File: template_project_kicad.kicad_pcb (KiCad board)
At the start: 2 copper layers, 53.3 x 50.8 mm, 5 parts

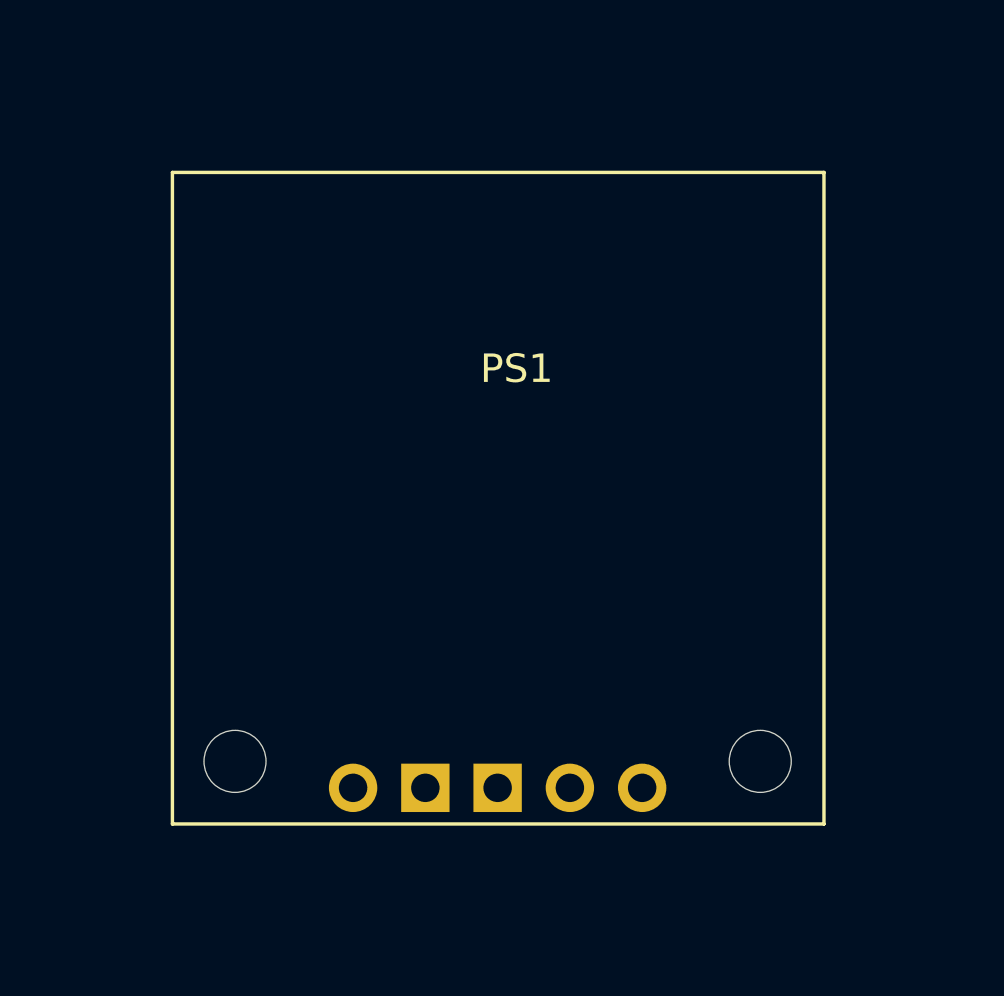
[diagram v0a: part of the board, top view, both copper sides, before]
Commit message: Forced minor change to trigger CICD
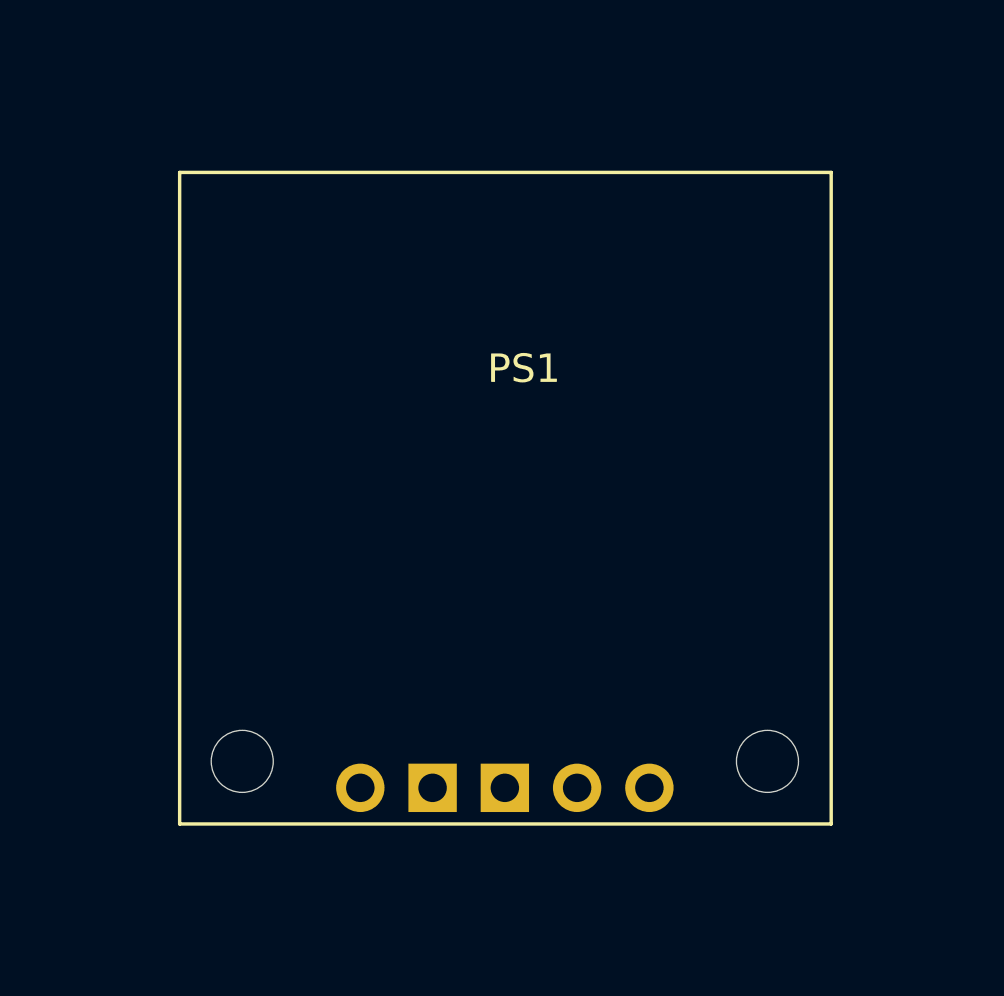
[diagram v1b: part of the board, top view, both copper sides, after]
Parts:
- moved PS1 0.25 mm to (115.9, 87.6)
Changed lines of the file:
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@@
   )
   (footprint "twyleg-voltage-regulators:Polulu-S13V30F5" (layer "F.Cu")
-    (at 115.645 87.555)
+    (at 115.899 87.555)
     (property "Sheetfile" "template_project_kicad.kicad_sch")
     (property "Sheetname" "")
